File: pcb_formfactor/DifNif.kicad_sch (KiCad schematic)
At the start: 27 parts, among them J2 PROG, J4 HPLA_PORT, U1 ICE40HX4K-TQ144, U13 Teensy4_1, U2 SST26VF080A-104I/SN, X1 ASE-xxxMHz

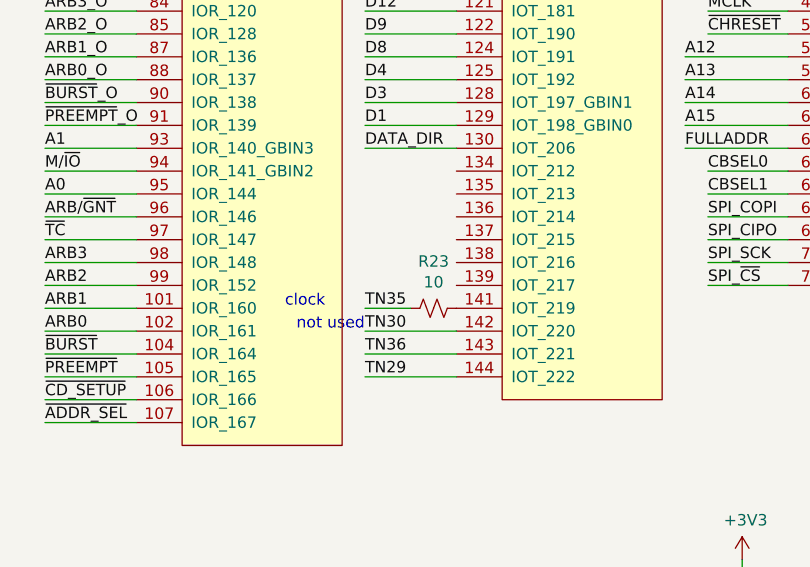
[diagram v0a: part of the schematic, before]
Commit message: fabout form factor pcb
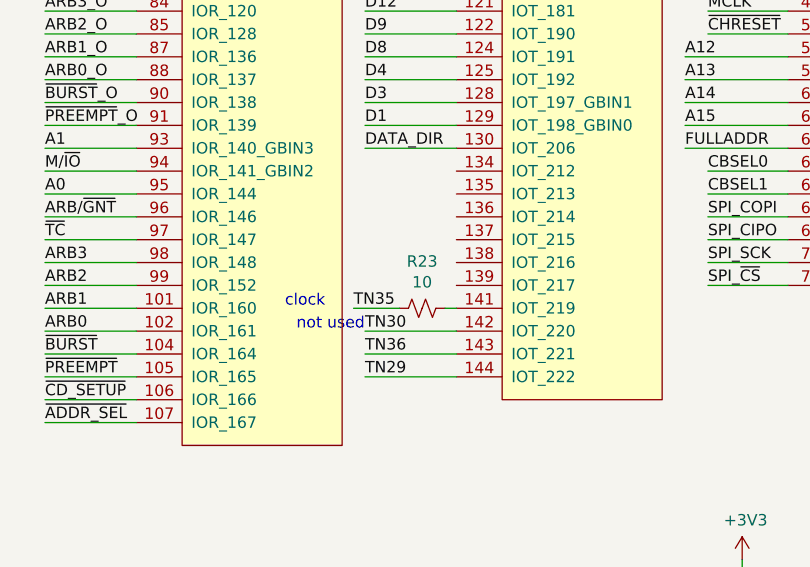
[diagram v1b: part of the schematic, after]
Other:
- moved on the sheet: R23
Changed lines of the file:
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@@
+    (stroke (width 0) (type default) (color 0 0 0 0))
+  )
+  (wire (pts (xy 115.57 121.92) (xy 116.84 121.92))
     (stroke (width 0) (type default) (color 0 0 0 0))
   )
@@
     (stroke (width 0) (type default) (color 0 0 0 0))
   )
-  (wire (pts (xy 106.68 121.92) (xy 111.76 121.92))
+  (wire (pts (xy 105.41 121.92) (xy 110.49 121.92))
     (stroke (width 0) (type default) (color 0 0 0 0))
   )
@@
     (effects (font (size 1.27 1.27)) (justify right bottom))
   )
-  (label "TN35" (at 106.68 121.92 0)
+  (label "TN35" (at 105.41 121.92 0)
     (effects (font (size 1.27 1.27)) (justify left bottom))
   )
@@
     (pin "2")
   )
-  (symbol (lib_id "Device:R_Small_US") (at 114.3 121.92 270) (unit 1)
-    (in_bom yes) (on_board yes)
-    (property "Reference" "R23" (id 0) (at 114.3 116.713 90))
-    (property "Value" "10" (id 1) (at 114.3 119.0244 90))
-    (property "Footprint" "Passive:RESC1608X55" (id 2) (at 114.3 121.92 0)
-      (effects (font (size 1.27 1.27)) hide)
-    )
-    (property "Datasheet" "~" (id 3) (at 114.3 121.92 0)
-      (effects (font (size 1.27 1.27)) hide)
-    )
-    (property "Mouser" "603-RC0603FR-0710RL" (id 4) (at 62.23 -6.35 0)
-      (effects (font (size 1.27 1.27)) hide)
-    )
+  (symbol (lib_id "Device:R_Small_US") (at 113.03 121.92 270) (unit 1)
+    (in_bom yes) (on_board yes)
+    (property "Reference" "R23" (id 0) (at 113.03 116.713 90))
+    (property "Value" "10" (id 1) (at 113.03 119.0244 90))
+    (property "Footprint" "Passive:RESC1608X55" (id 2) (at 113.03 121.92 0)
+      (effects (font (size 1.27 1.27)) hide)
+    )
+    (property "Datasheet" "~" (id 3) (at 113.03 121.92 0)
+      (effects (font (size 1.27 1.27)) hide)
+    )
+    (property "Mouser" "603-RC0603FR-0710RL" (id 4) (at 60.96 -6.35 0)
+      (effects (font (size 1.27 1.27)) hide)
+    )
